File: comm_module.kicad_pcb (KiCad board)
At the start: 4 copper layers, 112.4 x 100.1 mm, 74 parts, among them J1 USB-231-ARY, J2 PH2.54-01-03PZS, J3 U.FL-R-SMT-1(80), J4 U.FL-R-SMT-1(80), J5 U.FL-R-SMT-1(80), J6 U.FL-R-SMT-1(80), J7 S3B-ZR-SM4A-TF(LF)(SN), J8 SMN-305-ARP7, J9 U.FL-R-SMT-1(80), Q1 BSS138PW,115, U1 MIC29302WU, U2 SIM7600E, U3 TXU0202DCUR, U4 TCA9406DCUR, X1 WJ500V-5.08-2P-14-00A

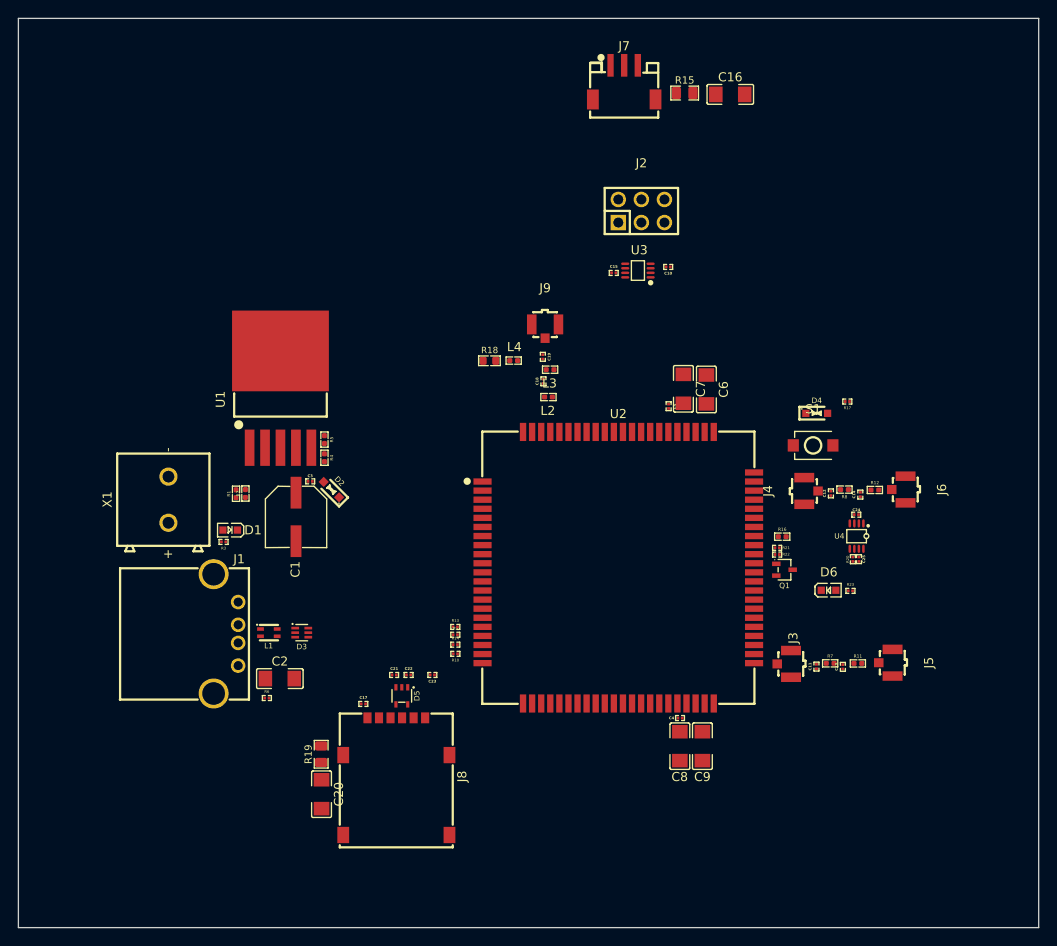
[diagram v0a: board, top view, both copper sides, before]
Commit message: First no error draft
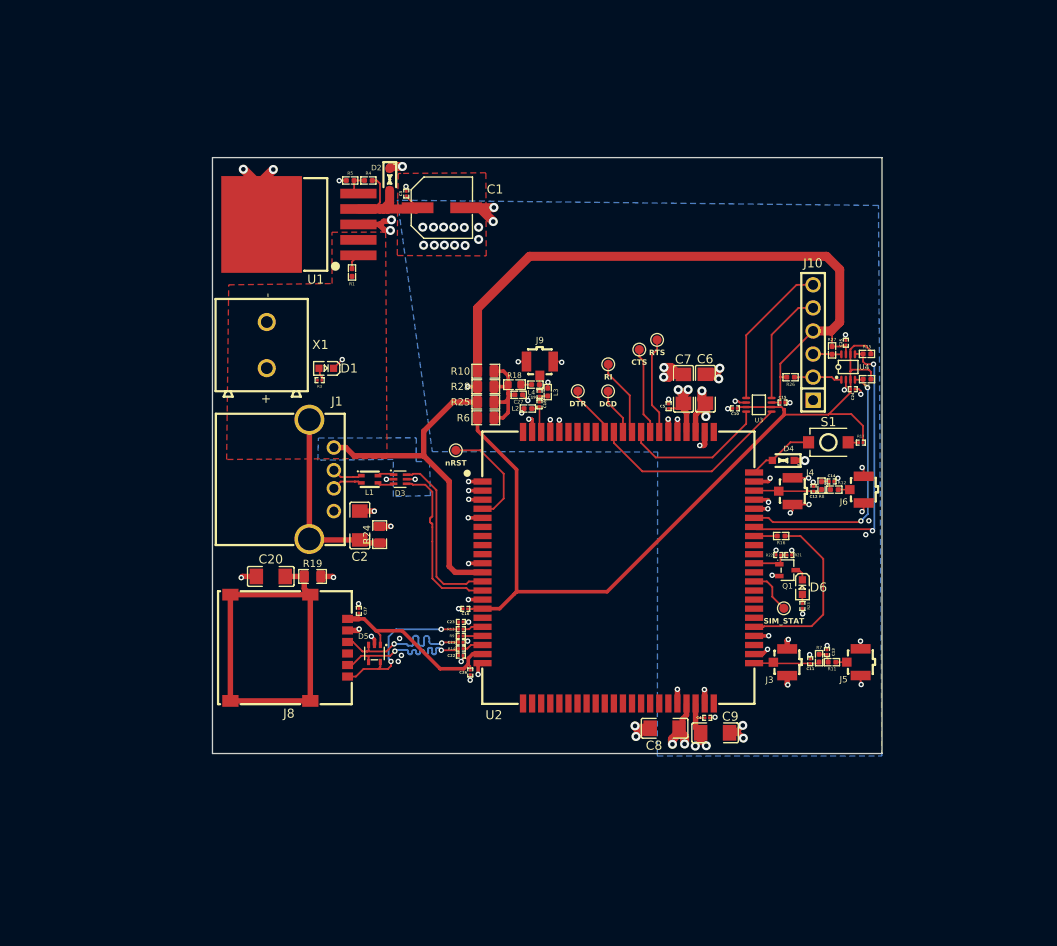
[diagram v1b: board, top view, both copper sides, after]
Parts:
- removed J2: PH2.54-01-03PZS, pepy_sym_lib:[2x3_PIN_HEADER_STR]XUNPU PH2.54-01-03PZS
- removed J7: S3B-ZR-SM4A-TF(LF)(SN), pepy_sym_lib:[JST_1X3P_1_5MM_R_ANGLE]JST S3B-ZR-SM4A-TF(LF)(SN)
- removed R20: 0201WMF1002TEE, pepy_sym_lib:[RES_SMD_0201_0603Metric]
- added C26: CC0201KRX5R6BB104, pepy_sym_lib:[CAP_SMD_0201_0603Metric], F.Cu at (79.7, 86.3)
- added C27: CC0402KRX7R7BB104, pepy_sym_lib:[CAP_SMD_0402_1005Metric], F.Cu at (85.1, 55.7)
- added J10: PZ254V-11-06P, pepy_sym_lib:[6P_HEADER_STR]XFCN PZ254V-11-06P, F.Cu at (117.5, 50.0)
- added R24: 0805W8F1004T5E, pepy_sym_lib:[RES_SMD_0805_2012Metric], F.Cu at (69.8, 71.1)
- added R25: 0805W8F0000T5E, pepy_sym_lib:[RES_SMD_0805_2012Metric], F.Cu at (81.5, 56.5)
- added R26: 0402WGF2201TCE, pepy_sym_lib:[RES_SMD_0402_1005Metric], F.Cu at (115.0, 53.8)
- added R27: 0402WGF2201TCE, pepy_sym_lib:[RES_SMD_0402_1005Metric], F.Cu at (119.6, 50.8)
- added R28: 0805W8F0000T5E, pepy_sym_lib:[RES_SMD_0805_2012Metric], F.Cu at (81.5, 54.8)
- added TP1: DCD, pepy_sym_lib:[TEST_POINT]TestPoint_Pad_D1.0mm, F.Cu at (94.9, 55.3)
- added TP2: RI, pepy_sym_lib:[TEST_POINT]TestPoint_Pad_D1.0mm, F.Cu at (94.9, 52.4)
- added TP3: DTR, pepy_sym_lib:[TEST_POINT]TestPoint_Pad_D1.0mm, F.Cu at (91.6, 55.3)
- added TP4: RTS, pepy_sym_lib:[TEST_POINT]TestPoint_Pad_D1.0mm, F.Cu at (100.3, 49.7)
- added TP5: CTS, pepy_sym_lib:[TEST_POINT]TestPoint_Pad_D1.0mm, F.Cu at (98.3, 50.7)
- added TP6: SIM_STAT, pepy_sym_lib:[TEST_POINT]TestPoint_Pad_D1.0mm, F.Cu at (114.3, 79.2)
- added TP7: nRST, pepy_sym_lib:[TEST_POINT]TestPoint_Pad_D1.0mm, F.Cu at (78.2, 61.8)
- C16: value CC1206KKX7RDBB102 -> CC0201KRX5R6BB104; footprint pepy_sym_lib:[CAP_SMD_1206_3216Metric] -> pepy_sym_lib:[CAP_SMD_0201_0603Metric]
- J3, J4, J5, J6, J9: value U.FL-R-SMT-1(80) -> U.FLRSMT1
- R10: value RC0201FR-0733RL -> 0805W8F0000T5E; footprint pepy_sym_lib:[RES_SMD_0201_0603Metric] -> pepy_sym_lib:[RES_SMD_0805_2012Metric]
- R15: value 0805W8F1004T5E -> 0402WGF2201TCE; footprint pepy_sym_lib:[RES_SMD_0805_2012Metric] -> pepy_sym_lib:[RES_SMD_0402_1005Metric]
- R2: value 0402WGF0000TCE -> 0402WGF2201TCE
- R6: value RC0201FR-071ML -> 0805W8F0000T5E; footprint pepy_sym_lib:[RES_SMD_0201_0603Metric] -> pepy_sym_lib:[RES_SMD_0805_2012Metric]
- moved R2 69.6 mm to (123.4, 54.0), turned to 0 degrees
- moved C16 63.7 mm to (79.2, 79.3)
- moved R6 39.2 mm to (81.5, 58.2), turned to 180 degrees
- moved C1 37.6 mm to (76.6, 35.1), turned to 0 degrees
- moved R15 35.0 mm to (123.4, 51.2)
- moved D2 34.7 mm to (70.9, 32.0), turned to -90 degrees
- moved C3 33.4 mm to (72.7, 33.5), turned to -90 degrees
- moved R10 31.3 mm to (81.5, 53.1)
- moved R4 30.9 mm to (68.5, 32.1), turned to 0 degrees
- moved R5 28.7 mm to (66.5, 32.1), turned to 0 degrees
- moved R1 27.5 mm to (66.7, 42.2)
- moved C20 24.6 mm to (57.8, 75.7), turned to 180 degrees
- moved C25 23.9 mm to (121.1, 50.0), turned to 90 degrees
- moved C15 23.4 mm to (114.1, 56.6), turned to 180 degrees
- moved D1 20.7 mm to (63.9, 52.8)
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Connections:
- net /D+_COMM renamed /DCOMM+
- net /D-_COMM renamed /DCOMM-
- net Net-(D3-I/O1-Pad1) renamed /DFILT-
- net Net-(D3-I/O2-Pad3) renamed /DFILT+
- C10 pad 2: VDD_3V3 -> /1V8_COMM
- C11 pad 2: Net-(C11-Pad2) -> /MAIN_ANT
- C12 pad 2: Net-(C12-Pad2) -> /AUX_ANT
- C15 pad 2: /1V8_COMM -> /VDD_3V3
- C16 pad 1: Earth_UART -> GND
- C16 pad 2: GND -> /1V8_COMM
- C25 pad 1: VDD_3V3 -> /VDD_3V3
- D5 pad 1: /SIM_DATA -> /SIM_VCC
- D5 pad 3: /SIM_VCC -> /SIM_RST
- D5 pad 4: /SIM_RST -> /SIM_CLK
- D5 pad 5: /SIM_CLK -> /SIM_DATA
- Q1 pad 1: /NETFLIGHT -> /NETLIGHT
- R10 pad 1: /SIM_VCC -> Net-(C27-Pad2)
- R10 pad 2: Net-(U2A-USIM_VDD) -> /VDD_3V3
- R15 pad 1: Earth_UART -> /COMM_SCL
- R15 pad 2: GND -> /1V8_COMM
- R16 pad 2: /1V8_COMM -> /VDD_AUX
- R18 pad 2: /SIM_VCC -> Net-(C27-Pad2)
- R2 pad 1: /EN -> /COMM_SDA
- R2 pad 2: Net-(U1-EN) -> /1V8_COMM
- R21 pad 2: /NETFLIGHT -> /NETLIGHT
- R22 pad 2: /NETFLIGHT -> /NETLIGHT
- R23 pad 2: VDD_3V3 -> /VDD_COMM
- R6 pad 1: Earth_USB -> Net-(C27-Pad2)
- R6 pad 2: GND -> /1V8_COMM
- R7 pad 1: Net-(C11-Pad2) -> /MAIN_ANT
- R8 pad 1: Net-(C12-Pad2) -> /AUX_ANT
- U2 pad 20: Net-(U2A-USIM_VDD) -> /SIM_VCC
- U2 pad 4: /nRST -> Net-(U2A-RESET)
- U2 pad 44: unconnected-(U2B-VDD_AUX-Pad44) -> /VDD_AUX
- U3 pad 1: /M_RX_S_TX_1V8 -> /M_TX_S_RX
- U3 pad 3: VDD_3V3 -> /1V8_COMM
- U3 pad 4: /M_RX_S_TX -> /M_TX_S_RX_1V8
- U3 pad 5: /M_TX_S_RX -> /M_RX_S_TX_1V8
- U3 pad 6: VDD_3V3 -> /1V8_COMM
- U3 pad 7: /1V8_COMM -> /VDD_3V3
- U3 pad 8: /M_TX_S_RX_1V8 -> /M_RX_S_TX
- U4 pad 6: Net-(U4-OE) -> /1V8_COMM
- U4 pad 7: VDD_3V3 -> /VDD_3V3
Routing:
- net GND: track 0.00 -> 118.3 mm, vias 0 -> 86
- net /1V8_COMM: track 0.00 -> 96.1 mm
- net /VDD_3V3: track 0.00 -> 74.4 mm
- net /VDD_COMM: track 0.00 -> 48.4 mm, vias 0 -> 22
- net Earth_SIM: track 0.00 -> 45.4 mm
- net /VBUS: track 0.00 -> 38.5 mm, vias 0 -> 1
- net /COMM_SCL: track 0.00 -> 34.7 mm, vias 0 -> 2
- net /COMM_SDA: track 0.00 -> 29.1 mm, vias 0 -> 2
- net /M_RX_S_TX_1V8: track 0.00 -> 22.6 mm
- net /SIM_VCC: track 0.00 -> 21.4 mm
- net Earth_USB: track 0.00 -> 21.1 mm
- net /VDD_AUX: track 0.00 -> 19.6 mm
- net /DCOMM-: track 0.00 -> 19.1 mm
- net /DCOMM+: track 0.00 -> 19.1 mm
- net /SIM_DATA: track 0.00 -> 18.3 mm, vias 0 -> 2
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- added copper zone on B.Cu, net /VBUS
- added copper zone on F.Cu, net /VBUS
- added copper zone on B.Cu, net /VDD_COMM
- added copper zone on F.Cu, net /VDD_COMM
- added copper zone on In1.Cu, net GND
- added copper zone on In2.Cu, net GND
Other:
- board size 112.4 x 100.1 mm -> 73.7 x 65.6 mm
- board text added: "0"
- board text added: "0 mm"
- board text added: "0.01 mm"
- board text added: "0.0152 mm"
- board text added: "0.02"
- board text added: "0.035 mm"
- board text added: "0.0994 mm"
- board text added: "1"
- board text added: "1.265 mm"
- board text added: "3.3"
- board text added: "4.1"
- board text added: "4.5"
- board text added: "B.Cu"
- board text added: "B.Mask"
- board text added: "B.Paste"
- board text added: "B.Silkscreen"
- board text added: "Bottom Silk Screen"
- board text added: "Bottom Solder Mask"
- board text added: "Bottom Solder Paste"
- board text added: "Color"
- board text added: "Dielectric"
- board text added: "Epsilon R"
- board text added: "F.Cu"
- board text added: "F.Mask"
- board text added: "F.Paste"
- board text added: "F.Silkscreen"
- board text added: "FR4"
- board text added: "In1.Cu"
- board text added: "In2.Cu"
- board text added: "Layer Name"
- board text added: "Loss Tangent"
- board text added: "Material"
- board text added: "Not specified"
- board text added: "Thickness (mm)"
- board text added: "Top Silk Screen"
- board text added: "Top Solder Mask"
- board text added: "Top Solder Paste"
- board text added: "Type"
- board text added: "copper"
- board text added: "core"
- board text added: "prepreg"
